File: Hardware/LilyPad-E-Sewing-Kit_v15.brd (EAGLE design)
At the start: 50.9 x 52.1 mm, 53 parts

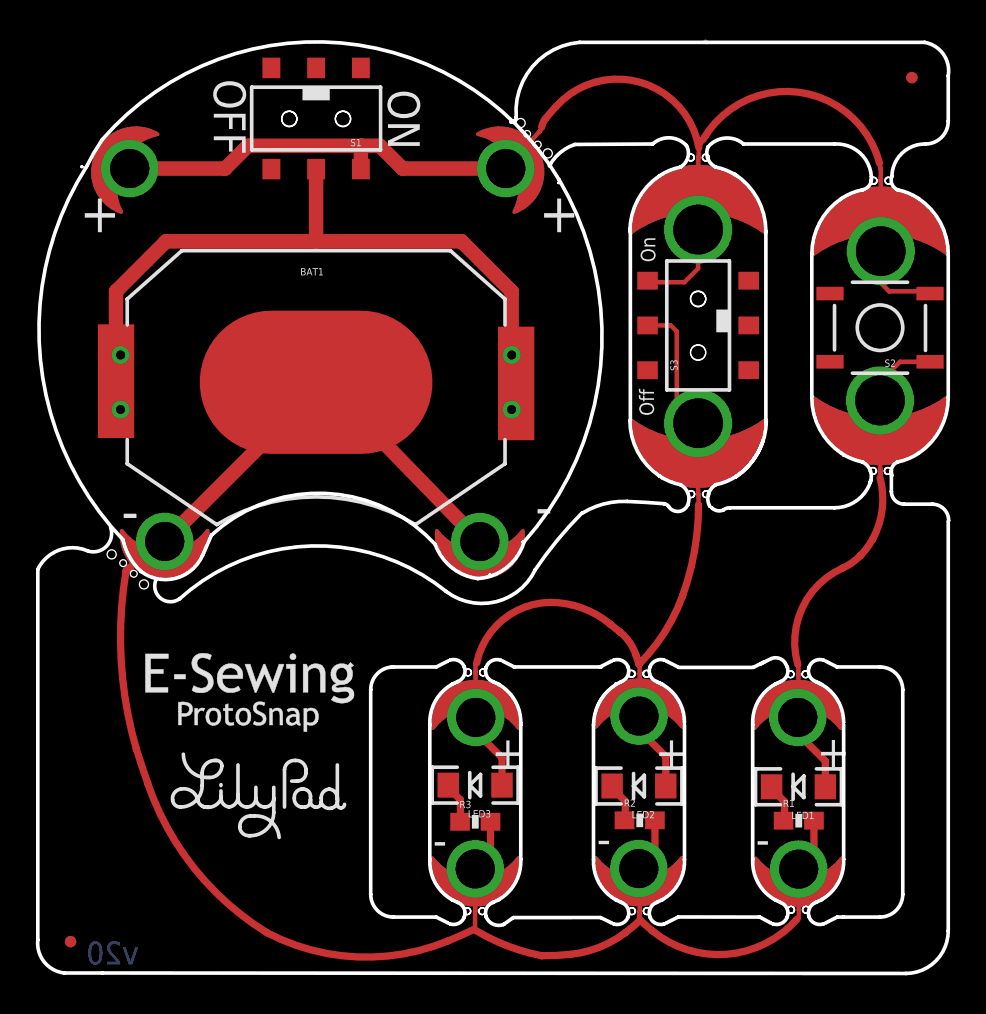
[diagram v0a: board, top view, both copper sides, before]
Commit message: Picked a different grid....
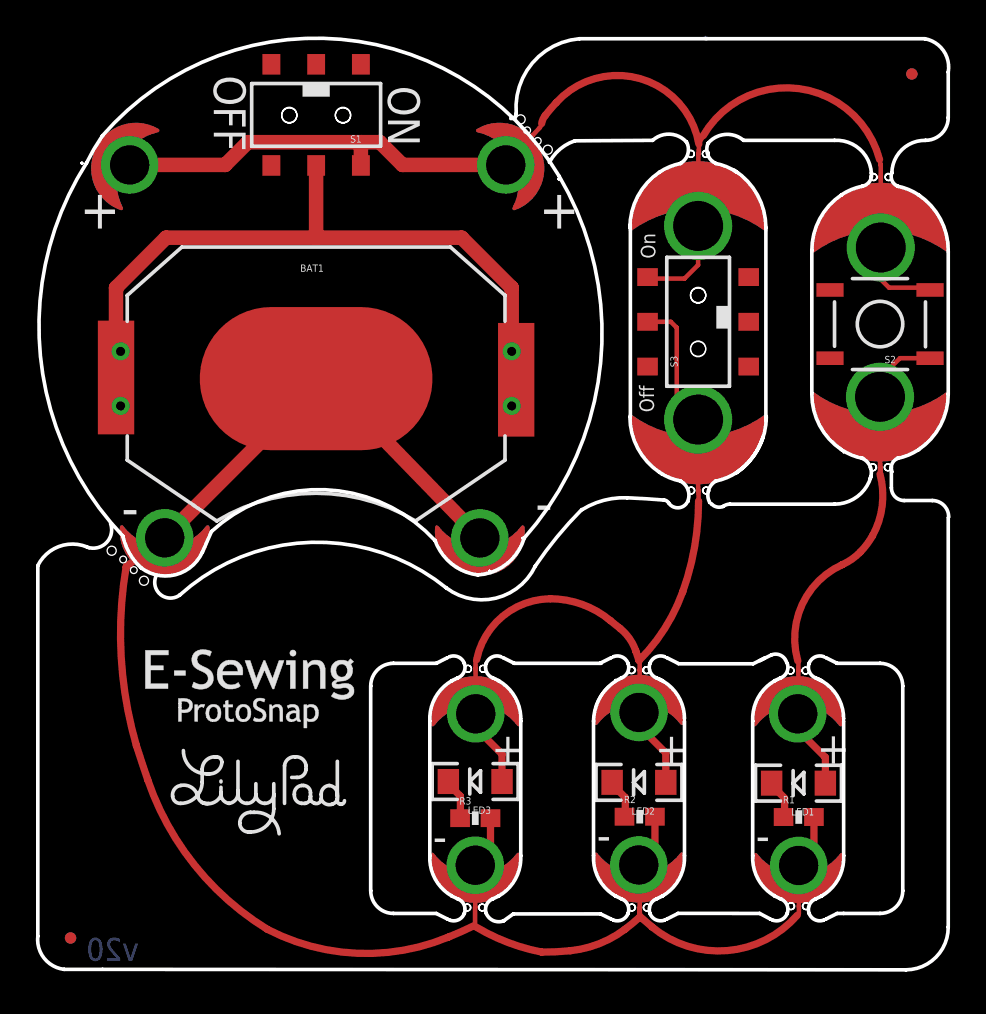
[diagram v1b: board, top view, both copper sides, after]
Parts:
- moved BAT1 0.20 mm to (15.5, 33.1)
- moved BATB-2 0.20 mm to (24.6, 24.2)
- moved BUTTON- 0.20 mm to (47.0, 40.2)
- moved BUTTONS 0.20 mm to (47.0, 32.3)
- moved LOGO1 0.20 mm to (11.0, 46.6)
- moved MB2 0.20 mm to (47.0, 44.4)
- moved MB4 0.20 mm to (33.6, 16.8)
- moved S1 0.20 mm to (15.5, 47.8)
- moved S3 0.20 mm to (36.8, 36.3)
- moved SLIDEON 0.20 mm to (36.8, 41.4)
- moved U$3 0.20 mm to (15.3, 36.7)
- moved U$5 0.20 mm to (36.3, 35.7)
- moved U$6 0.20 mm to (46.0, 35.7)
- moved LED+1 0.20 mm to (42.4, 14.4)
- moved LED+2 0.20 mm to (33.5, 14.5)
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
